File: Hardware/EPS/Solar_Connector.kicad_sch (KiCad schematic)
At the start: 4 parts

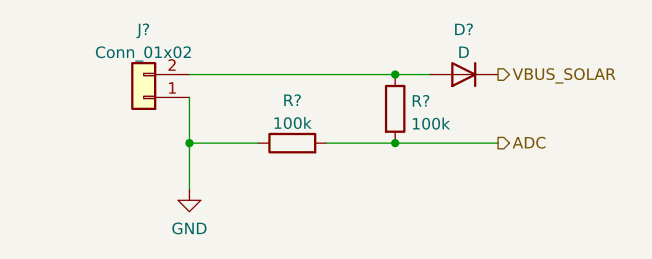
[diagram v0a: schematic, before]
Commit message: EPS v0.0.1
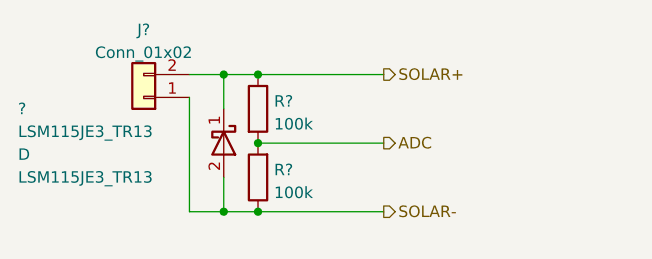
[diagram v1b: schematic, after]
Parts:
- removed D?: D, symbol Device:D
- removed R?: 100k, symbol Device:R
- added ?: LSM115JE3_TR13, symbol LSM115JE3_TR13:LSM115JE3_TR13
- added R?: 100k, symbol Device:R
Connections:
- net ADC: now also R?.2
- net SOLAR+: now reaches J?.2 (Pin_2), R?.1
- net SOLAR+: now also ?.1 (K)
- net GND renamed SOLAR-
- net SOLAR-: now also ?.2 (A), R?.1
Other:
- moved on the sheet: R?
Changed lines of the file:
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@@
 (kicad_sch (version 20211123) (generator eeschema)
   (paper "A4")
-  (junction (at 138.43 82.55) (diameter 0) (color 0 0 0 0)
+  (junction (at 123.19 90.17) (diameter 0) (color 0 0 0 0)
   )
-  (junction (at 115.57 82.55) (diameter 0) (color 0 0 0 0)
+  (junction (at 123.19 82.55) (diameter 0) (color 0 0 0 0)
   )
-  (junction (at 138.43 74.93) (diameter 0) (color 0 0 0 0)
+  (junction (at 119.38 90.17) (diameter 0) (color 0 0 0 0)
   )
-  (wire (pts (xy 130.81 82.55) (xy 138.43 82.55))
+  (junction (at 119.38 74.93) (diameter 0) (color 0 0 0 0)
+  )
+  (junction (at 123.19 74.93) (diameter 0) (color 0 0 0 0)
+  )
+  (wire (pts (xy 123.19 82.55) (xy 137.16 82.55))
     (stroke (width 0) (type default) (color 0 0 0 0))
   )
-  (wire (pts (xy 138.43 82.55) (xy 149.86 82.55))
+  (wire (pts (xy 115.57 77.47) (xy 115.57 90.17))
     (stroke (width 0) (type default) (color 0 0 0 0))
   )
-  (wire (pts (xy 115.57 87.63) (xy 115.57 82.55))
+  (wire (pts (xy 119.38 86.36) (xy 119.38 90.17))
     (stroke (width 0) (type default) (color 0 0 0 0))
   )
-  (wire (pts (xy 115.57 82.55) (xy 115.57 77.47))
+  (wire (pts (xy 119.38 74.93) (xy 123.19 74.93))
     (stroke (width 0) (type default) (color 0 0 0 0))
   )
-  (wire (pts (xy 123.19 82.55) (xy 115.57 82.55))
+  (wire (pts (xy 115.57 90.17) (xy 119.38 90.17))
     (stroke (width 0) (type default) (color 0 0 0 0))
   )
-  (wire (pts (xy 138.43 74.93) (xy 142.24 74.93))
+  (wire (pts (xy 123.19 74.93) (xy 137.16 74.93))
     (stroke (width 0) (type default) (color 0 0 0 0))
   )
-  (wire (pts (xy 115.57 74.93) (xy 138.43 74.93))
+  (wire (pts (xy 119.38 74.93) (xy 119.38 78.74))
     (stroke (width 0) (type default) (color 0 0 0 0))
   )
-  (hierarchical_label "VBUS_SOLAR" (shape output) (at 149.86 74.93 0)
+  (wire (pts (xy 115.57 74.93) (xy 119.38 74.93))
+    (stroke (width 0) (type default) (color 0 0 0 0))
+  )
+  (wire (pts (xy 123.19 90.17) (xy 137.16 90.17))
+    (stroke (width 0) (type default) (color 0 0 0 0))
+  )
+  (wire (pts (xy 119.38 90.17) (xy 123.19 90.17))
+    (stroke (width 0) (type default) (color 0 0 0 0))
+  )
+  (hierarchical_label "SOLAR-" (shape output) (at 137.16 90.17 0)
     (effects (font (size 1.27 1.27)) (justify left))
   )
-  (hierarchical_label "ADC" (shape output) (at 149.86 82.55 0)
+  (hierarchical_label "SOLAR+" (shape output) (at 137.16 74.93 0)
     (effects (font (size 1.27 1.27)) (justify left))
   )
-  (symbol (lib_id "Device:R") (at 138.43 78.74 0) (unit 1)
+  (hierarchical_label "ADC" (shape output) (at 137.16 82.55 0)
+    (effects (font (size 1.27 1.27)) (justify left))
+  )
+  (symbol (lib_id "Device:R") (at 123.19 78.74 0) (unit 1)
     (in_bom yes) (on_board yes) (fields_autoplaced)
-    (property "Reference" "R?" (id 0) (at 140.208 77.9053 0)
+    (property "Reference" "R?" (id 0) (at 124.968 77.9053 0)
       (effects (font (size 1.27 1.27)) (justify left))
     )
-    (property "Value" "100k" (id 1) (at 140.208 80.4422 0)
+    (property "Value" "100k" (id 1) (at 124.968 80.4422 0)
       (effects (font (size 1.27 1.27)) (justify left))
     )
-    (property "Footprint" "" (id 2) (at 136.652 78.74 90)
+    (property "Footprint" "" (id 2) (at 121.412 78.74 90)
       (effects (font (size 1.27 1.27)) hide)
     )
-    (property "Datasheet" "~" (id 3) (at 138.43 78.74 0)
+    (property "Datasheet" "~" (id 3) (at 123.19 78.74 0)
       (effects (font (size 1.27 1.27)) hide)
     )
@@
     (pin "2")
   )
-  (symbol (lib_id "Device:D") (at 146.05 74.93 180) (unit 1)
+  (symbol (lib_id "Device:R") (at 123.19 86.36 180) (unit 1)
     (in_bom yes) (on_board yes) (fields_autoplaced)
-    (property "Reference" "D?" (id 0) (at 146.05 69.9602 0))
-    (property "Value" "D" (id 1) (at 146.05 72.4971 0))
-    (property "Footprint" "" (id 2) (at 146.05 74.93 0)
+    (property "Reference" "R?" (id 0) (at 124.968 85.5253 0)
+      (effects (font (size 1.27 1.27)) (justify right))
+    )
+    (property "Value" "100k" (id 1) (at 124.968 88.0622 0)
+      (effects (font (size 1.27 1.27)) (justify right))
+    )
+    (property "Footprint" "" (id 2) (at 124.968 86.36 90)
       (effects (font (size 1.27 1.27)) hide)
     )
-    (property "Datasheet" "~" (id 3) (at 146.05 74.93 0)
+    (property "Datasheet" "~" (id 3) (at 123.19 86.36 0)
       (effects (font (size 1.27 1.27)) hide)
     )
@@
     (pin "2")
   )
-  (symbol (lib_id "power:GND") (at 115.57 87.63 0) (unit 1)
-    (in_bom yes) (on_board yes) (fields_autoplaced)
-    (property "Reference" "#PWR?" (id 0) (at 115.57 93.98 0)
+  (symbol (lib_id "LSM115JE3_TR13:LSM115JE3_TR13") (at 119.38 82.55 270) (unit 1)
+    (in_bom yes) (on_board yes)
+    (property "Reference" "?" (id 0) (at 96.52 78.7431 90)
+      (effects (font (size 1.27 1.27)) (justify left))
+    )
+    (property "Value" "LSM115JE3_TR13" (id 1) (at 96.52 81.28 90)
+      (effects (font (size 1.27 1.27)) (justify left))
+    )
+    (property "Footprint" "" (id 2) (at 119.38 82.55 0)
       (effects (font (size 1.27 1.27)) hide)
     )
-    (property "Value" "GND" (id 1) (at 115.57 92.0734 0))
-    (property "Footprint" "" (id 2) (at 115.57 87.63 0)
+    (property "Datasheet" "" (id 3) (at 119.38 82.55 0)
       (effects (font (size 1.27 1.27)) hide)
     )
-    (property "Datasheet" "" (id 3) (at 115.57 87.63 0)
-      (effects (font (size 1.27 1.27)) hide)
+    (property "Reference_1" "D" (id 4) (at 96.52 83.8169 90)
+      (effects (font (size 1.27 1.27)) (justify left))
+    )
+    (property "Value_1" "LSM115JE3_TR13" (id 5) (at 96.52 86.3538 90)
+      (effects (font (size 1.27 1.27)) (justify left))
+    )
+    (property "Footprint_1" "DIOM5436X330N" (id 6) (at 25.73 95.25 0)
+      (effects (font (size 1.27 1.27)) (justify left top) hide)
+    )
+    (property "Datasheet_1" "https://media.digikey.com/pdf/Data%20Sheets/Microsemi%20PDFs/LSM115J.pdf" (id 7) (at -74.27 95.25 0)
+      (effects (font (size 1.27 1.27)) (justify left top) hide)
+    )
+    (property "Height" "3.3" (id 8) (at -274.27 95.25 0)
+      (effects (font (size 1.27 1.27)) (justify left top) hide)
+    )
+    (property "Manufacturer_Name" "Microsemi Corporation" (id 9) (at -374.27 95.25 0)
+      (effects (font (size 1.27 1.27)) (justify left top) hide)
+    )
+    (property "Manufacturer_Part_Number" "LSM115JE3/TR13" (id 10) (at -474.27 95.25 0)
+      (effects (font (size 1.27 1.27)) (justify left top) hide)
+    )
+    (property "Mouser Part Number" "494-LSM115JE3/TR13" (id 11) (at -574.27 95.25 0)
+      (effects (font (size 1.27 1.27)) (justify left top) hide)
+    )
+    (property "Mouser Price/Stock" "https://www.mouser.co.uk/ProductDetail/Microchip-Microsemi/LSM115JE3-TR13/?qs=6jAvgNDGUA8H9k1qUsKdHA%3D%3D" (id 12) (at -674.27 95.25 0)
+      (effects (font (size 1.27 1.27)) (justify left top) hide)
+    )
+    (property "Arrow Part Number" "LSM115JE3/TR13" (id 13) (at -774.27 95.25 0)
+      (effects (font (size 1.27 1.27)) (justify left top) hide)
+    )
+    (property "Arrow Price/Stock" "https://www.arrow.com/en/products/lsm115je3tr13/microsemi" (id 14) (at -874.27 95.25 0)
+      (effects (font (size 1.27 1.27)) (justify left top) hide)
     )
     (pin "1")
-  )
-  (symbol (lib_id "Device:R") (at 127 82.55 90) (unit 1)
-    (in_bom yes) (on_board yes) (fields_autoplaced)
-    (property "Reference" "R?" (id 0) (at 127 77.8342 90))
-    (property "Value" "100k" (id 1) (at 127 80.3711 90))
-    (property "Footprint" "" (id 2) (at 127 84.328 90)
-      (effects (font (size 1.27 1.27)) hide)
-    )
-    (property "Datasheet" "~" (id 3) (at 127 82.55 0)
-      (effects (font (size 1.27 1.27)) hide)
-    )
-    (pin "1")
